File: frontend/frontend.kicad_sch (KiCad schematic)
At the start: 24 parts, among them U1 ADG722, U2 ADG722, U3 OPA2387DGKT, U4 LM358

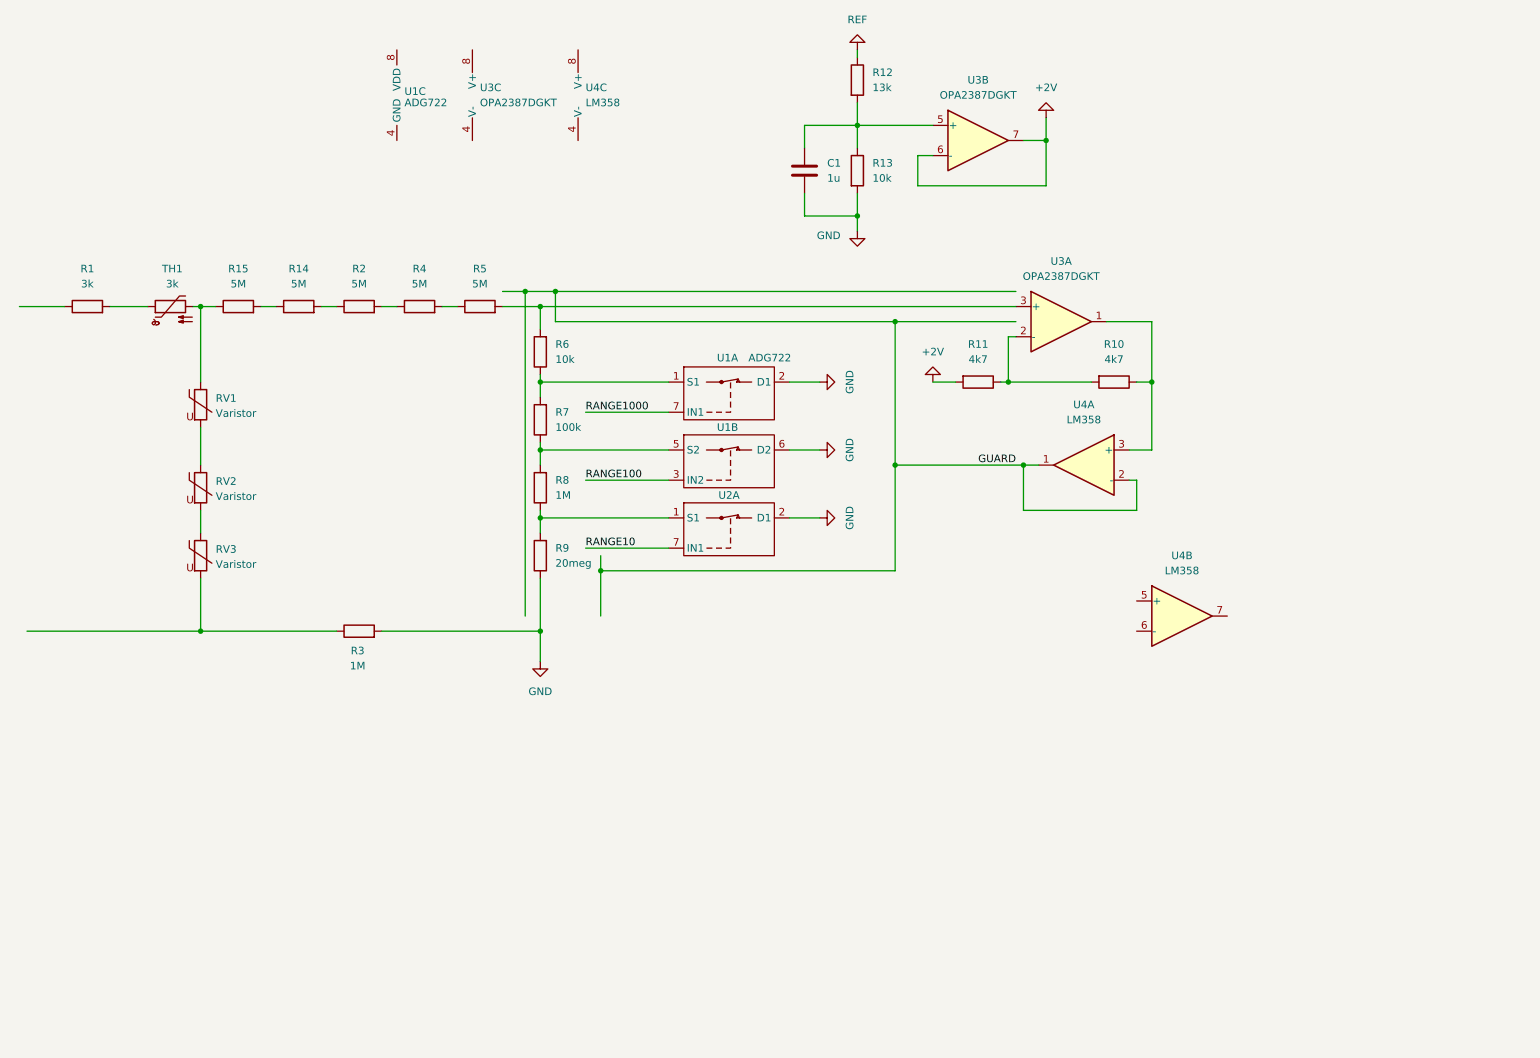
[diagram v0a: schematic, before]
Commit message: 2
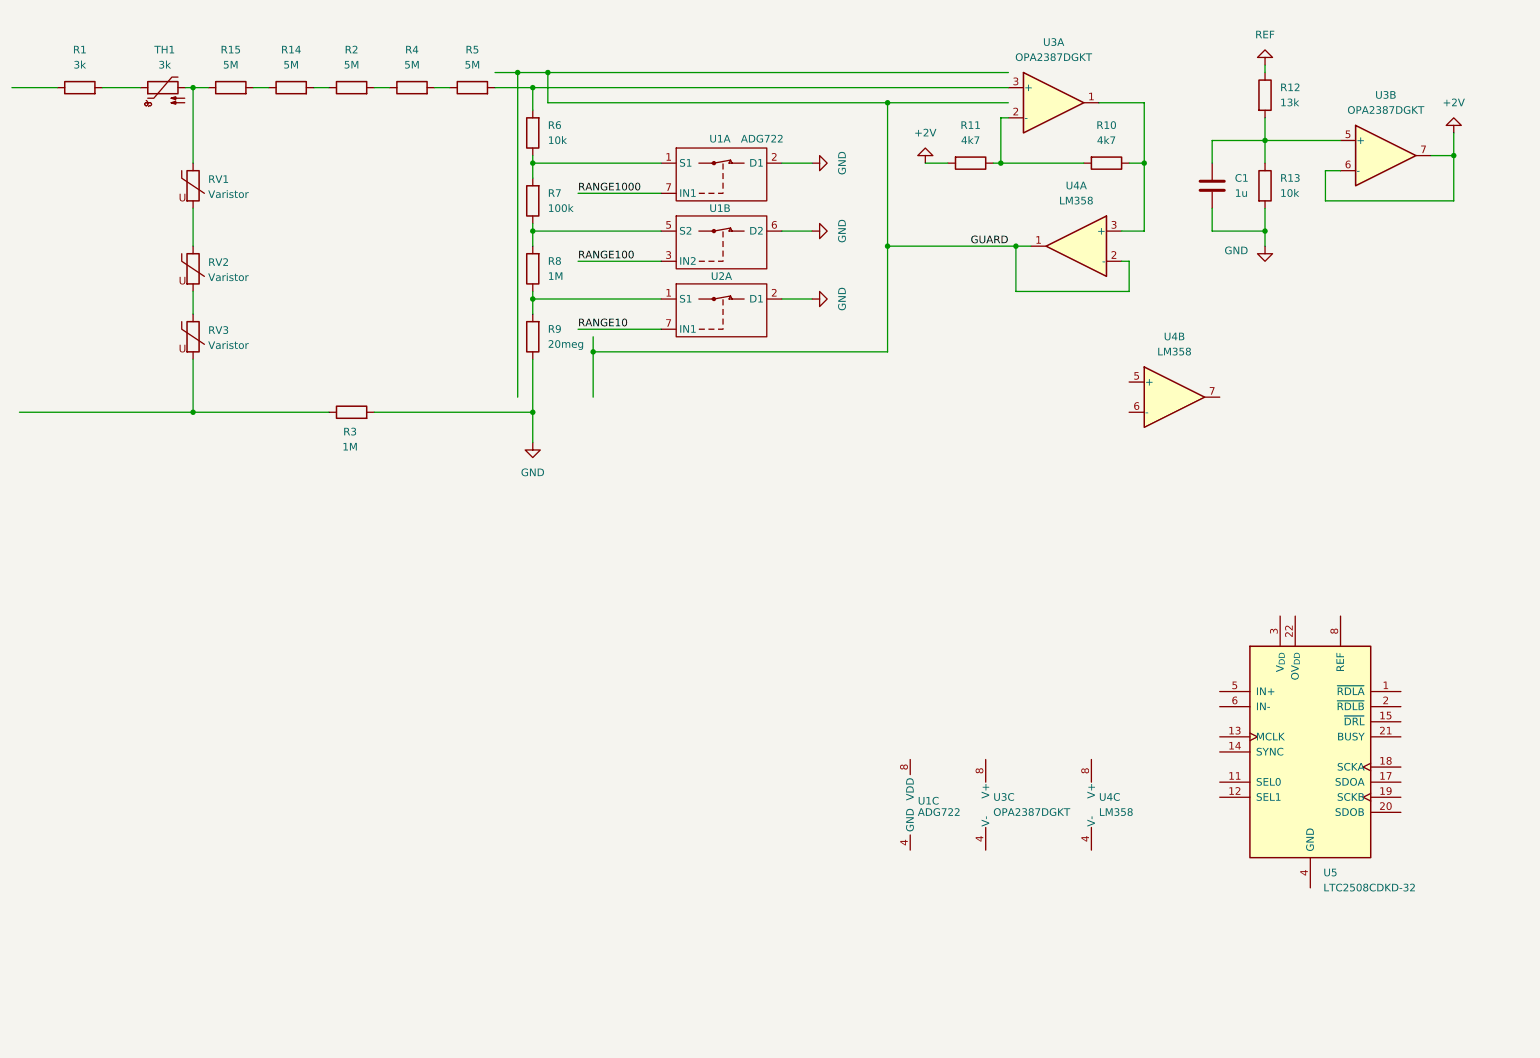
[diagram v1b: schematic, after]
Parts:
- added U5: LTC2508CDKD-32, Package_DFN_QFN:DFN-24-1EP_4x7mm_P0.5mm_EP2.64x6.44mm, symbol Analog_ADC:LTC2508CDKD-32
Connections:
- new net: U5.10 (REF), U5.8 (REF), U5.9 (REF)
- new net: U5.16 (GND), U5.23 (GND), U5.24 (GND), U5.25 (GND), U5.4 (GND), U5.7 (GND)
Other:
- moved on the sheet: C1, R1, R10, R11, R12, R13, R14, R15, R2, R3, R4, R5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

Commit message: 3
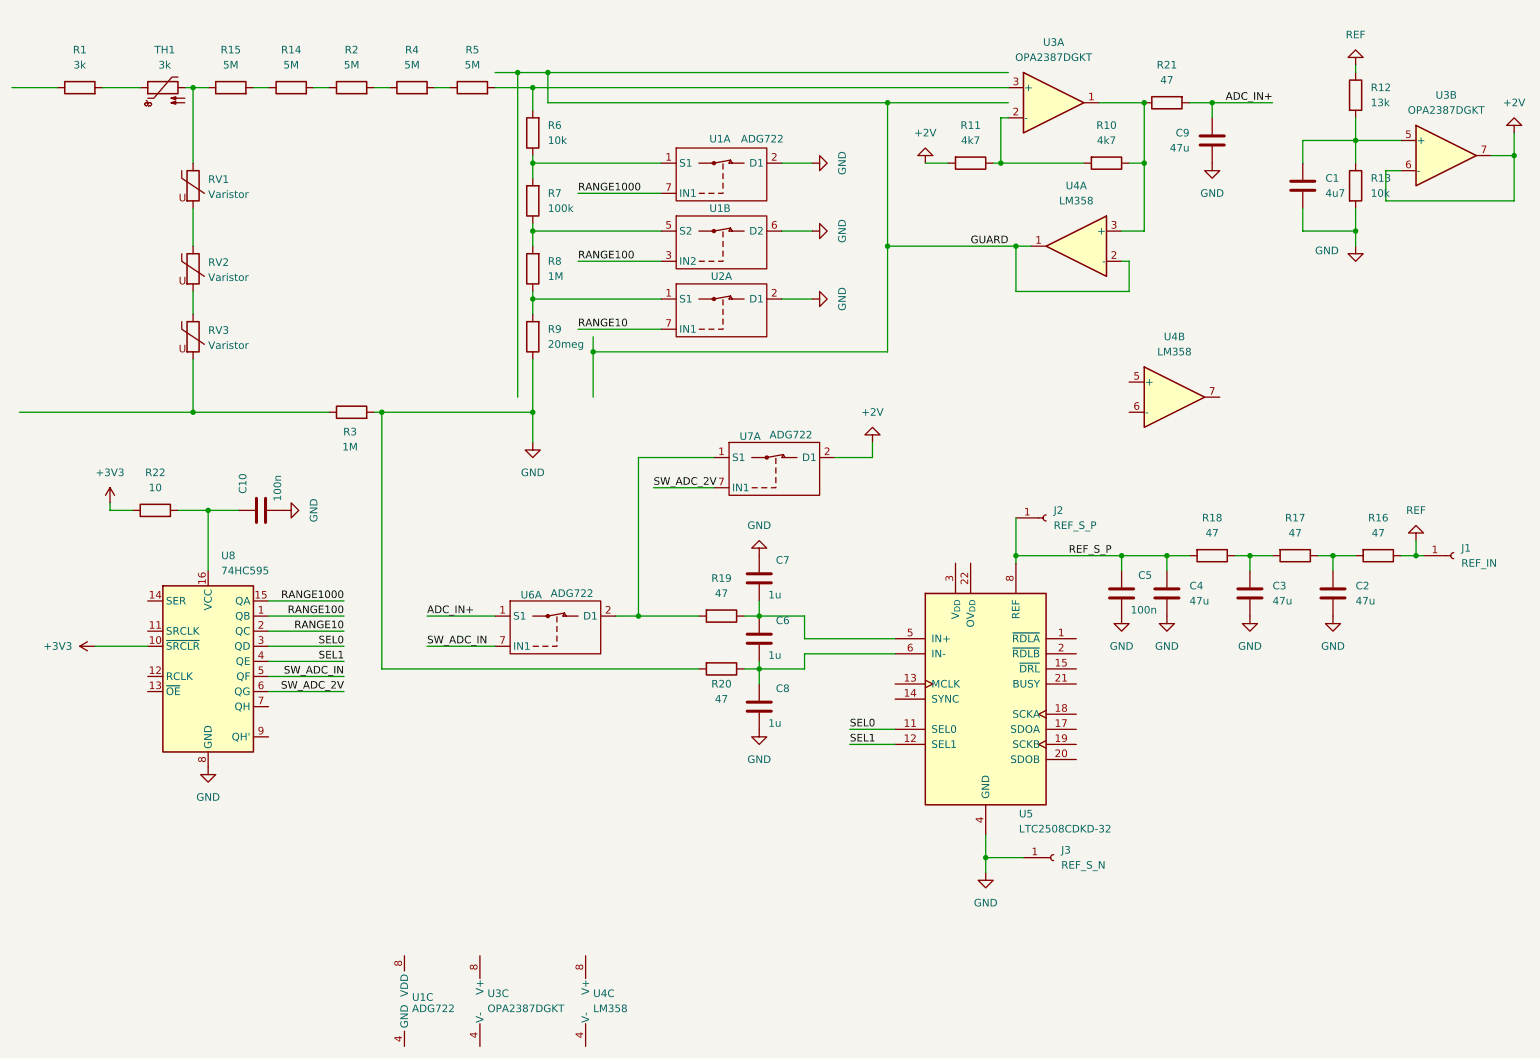
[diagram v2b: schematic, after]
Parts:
- added C10, C5: 100n, Capacitor_SMD:C_0805_2012Metric_Pad1.18x1.45mm_HandSolder, symbol Device:C
- added C2, C3, C4, C9: 47u, Capacitor_SMD:C_0805_2012Metric_Pad1.18x1.45mm_HandSolder, symbol Device:C
- added C6, C7, C8: 1u, Capacitor_SMD:C_0805_2012Metric_Pad1.18x1.45mm_HandSolder, symbol Device:C
- added J1: REF_IN, Connector_PinHeader_2.54mm:PinHeader_1x01_P2.54mm_Vertical, symbol Connector:Conn_01x01_Socket
- added J2: REF_S_P, Connector_PinHeader_2.54mm:PinHeader_1x01_P2.54mm_Vertical, symbol Connector:Conn_01x01_Socket
- added J3: REF_S_N, Connector_PinHeader_2.54mm:PinHeader_1x01_P2.54mm_Vertical, symbol Connector:Conn_01x01_Socket
- added R16, R17, R18, R19, R20, R21: 47, Resistor_SMD:R_1206_3216Metric_Pad1.30x1.75mm_HandSolder, symbol Device:R
- added R22: 10, Resistor_THT:R_Axial_DIN0207_L6.3mm_D2.5mm_P15.24mm_Horizontal, symbol Device:R
- added U6, U7: ADG722, Library:uSOIC, symbol New_Library:ADG722
- added U8: 74HC595, Package_SO:SOIC-16_3.9x9.9mm_P1.27mm, symbol 74xx:74HC595
- C1: value 1u -> 4u7
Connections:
- net +2V: now also U7.2 (D1)
- net GND: now also U5.16 (GND), U5.23 (GND), U5.24 (GND), U5.25 (GND), U5.4 (GND), U5.7 (GND), C10.2, C2.2, C3.2, C4.2, C5.2, C7.1, C8.2, C9.2, J3.1 (Pin_1), R20.2, U8.8 (GND)
- net RANGE10: now also U8.2 (QC)
- net RANGE100: now also U8.1 (QB)
- net RANGE1000: now also U8.15 (QA)
- net REF: now also J1.1 (Pin_1), R16.1
- net at R10.1, U3.1, U4.3 (+): now also R21.1
- net REF_S_P: now reaches U5.10 (REF), U5.8 (REF), U5.9 (REF)
- net REF_S_P: now also C4.1, C5.1, J2.1 (Pin_1), R18.2
- net SEL0: now reaches U5.11 (SEL0)
- net SEL0: now also U8.3 (QD)
- net SEL1: now reaches U5.12 (SEL1)
- net SEL1: now also U8.4 (QE)
- net at U5.5 (IN+): now also C6.1, C7.2, R19.1
- net at U5.6 (IN-): now also C6.2, C8.1, R20.1
- new net: C2.1, R16.2, R17.1
- new net: C3.1, R17.2, R18.1
- new net: R19.2, U6.2 (D1), U7.1 (S1)
- new net: C10.1, R22.2, U8.16 (VCC)
- new net +3V3: R22.1, U8.10 (~{SRCLR})
- new net ADC_IN+: C9.1, R21.2, U6.1 (S1)
- new net SW_ADC_2V: U7.7 (IN1), U8.6 (QG)
- new net SW_ADC_IN: U6.7 (IN1), U8.5 (QF)
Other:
- moved on the sheet: C1, R12, R13, U1C, U3B, U3C, U4C, U5
